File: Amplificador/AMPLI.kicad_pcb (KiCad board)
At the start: 2 copper layers, 46.8 x 32 mm, 18 parts, among them J2 Screw_Terminal_01x02, J3 Screw_Terminal_01x02, SW1 SW_DPST_x2, U1 TDA2050

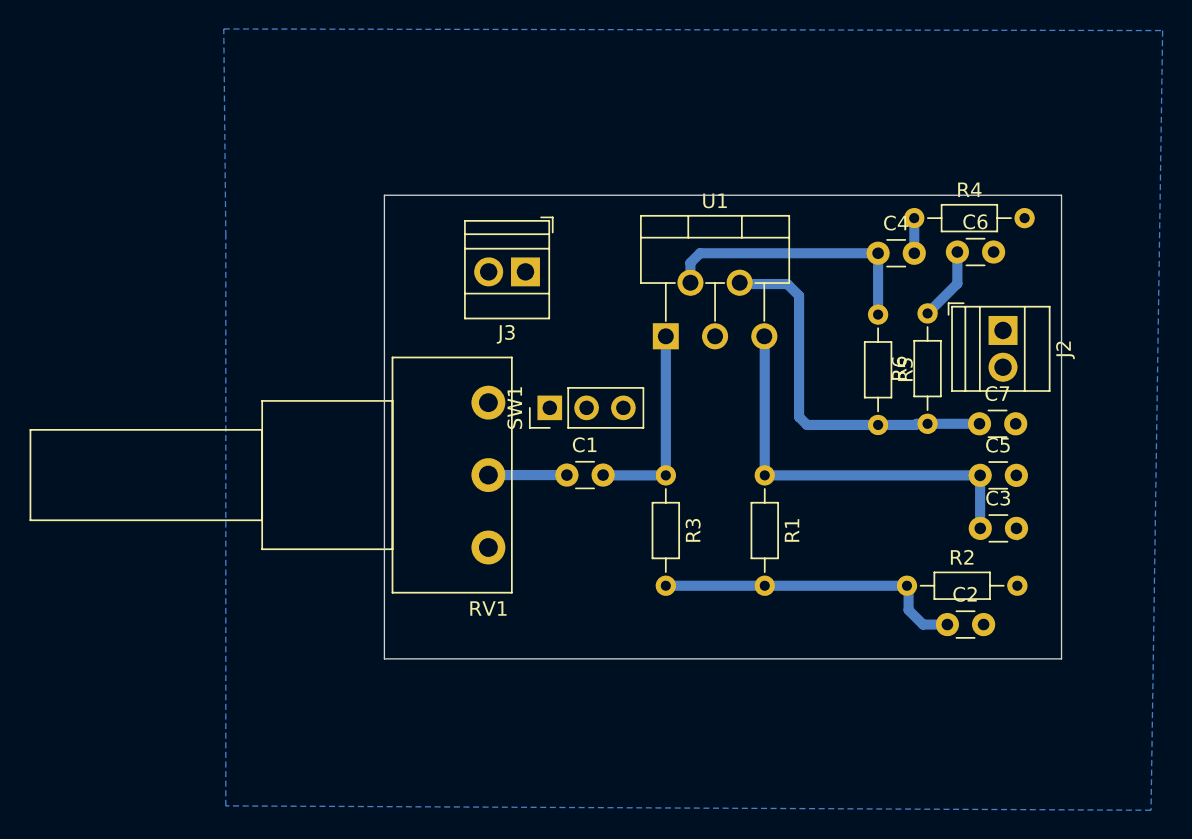
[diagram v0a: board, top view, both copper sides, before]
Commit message: commit20
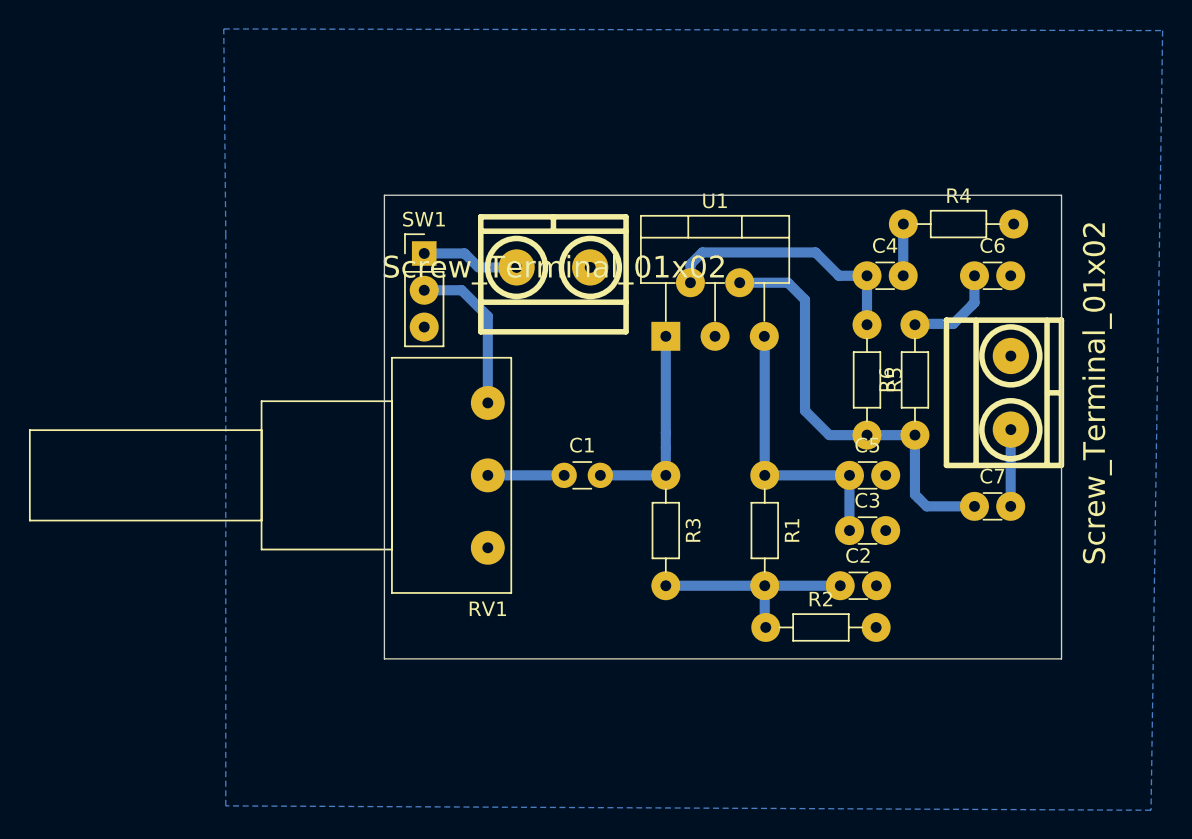
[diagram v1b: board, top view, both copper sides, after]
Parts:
- J2, J3: footprint TerminalBlock:TerminalBlock_Xinya_XY308-2.54-2P_1x02_P2.54mm_Horizontal -> EESTN5:BORNERA2_AZUL
- moved SW1 13.7 mm to (139.7, 88.9), turned to 0 degrees
- moved R2 10.2 mm to (163.3, 114.7)
- moved C3 9.03 mm to (169.1, 108.0)
- moved C5 9.02 mm to (169.1, 104.2)
- moved C2 7.87 mm to (168.4, 111.8)
- moved C7 5.71 mm to (177.7, 106.4)
- moved J2 4.34 mm to (180.2, 98.5), turned to 90 degrees
- moved C6 2.02 mm to (177.7, 90.5)
- moved J3 1.95 mm to (148.6, 89.9)
- moved C4 1.73 mm to (170.3, 90.5)
- moved R6 1.17 mm to (173.6, 101.5)
- moved R5 1.04 mm to (170.3, 93.8)
- moved R4 0.85 mm to (172.8, 86.9)
- moved C1 0.19 mm to (149.3, 104.2)
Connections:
- J3 pad 2: Net-(J1-Pin_1) -> Net-(J3-Pin_2)
- RV1 pad 1: Net-(J1-Pin_3) -> Net-(SW1A-B)
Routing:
- net Net-(SW1A-B): track 0.00 -> 11.1 mm
- net VCC: track 28.2 -> 19.3 mm
- net Net-(C2-Pad1): track 21.8 -> 14.9 mm
- net Net-(J3-Pin_2): track 0.00 -> 6.78 mm
- net Net-(J2-Pin_1): track 0.00 -> 5.30 mm
- net Net-(C7-Pad1): track 25.6 -> 29.5 mm
- net Net-(C6-Pad1): track 5.09 -> 6.60 mm
- net Net-(C4-Pad2): track 2.43 -> 3.57 mm
- net Net-(U1--): track 18.8 -> 17.8 mm
